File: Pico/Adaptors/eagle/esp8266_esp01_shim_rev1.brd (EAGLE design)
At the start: 17.1 x 10.7 mm, 4 parts, among them IC2 78L 3.3v

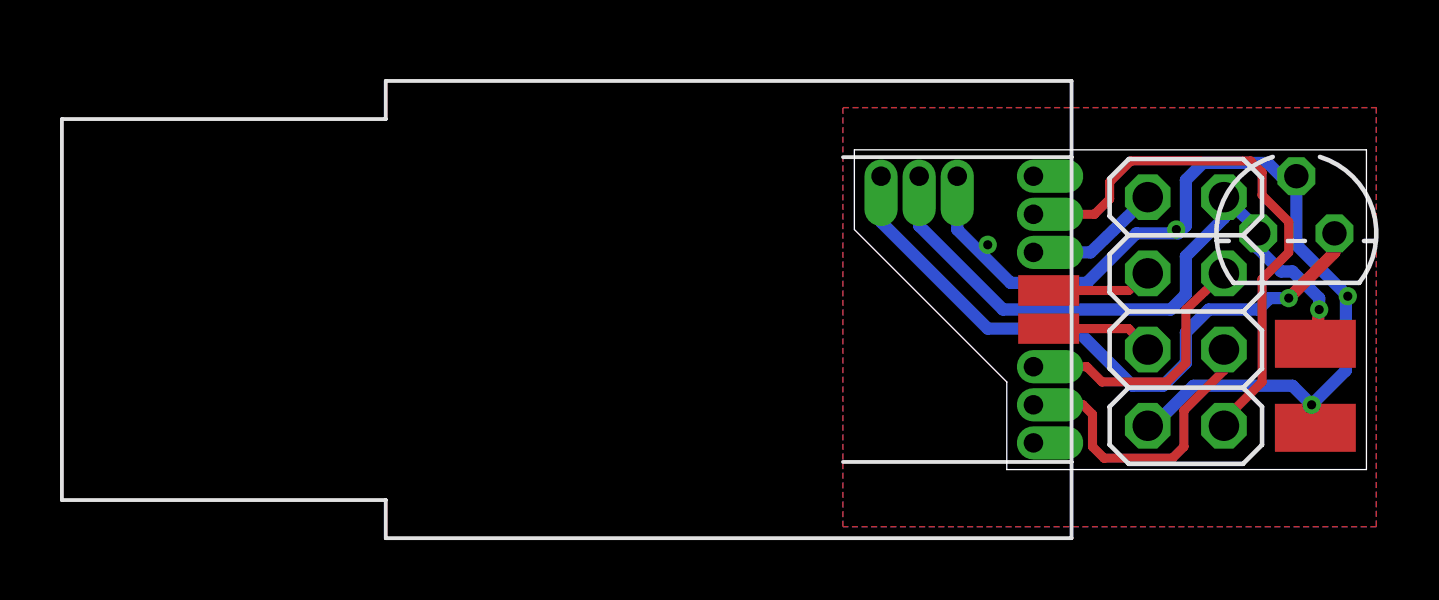
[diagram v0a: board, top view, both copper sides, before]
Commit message: tweak net classes
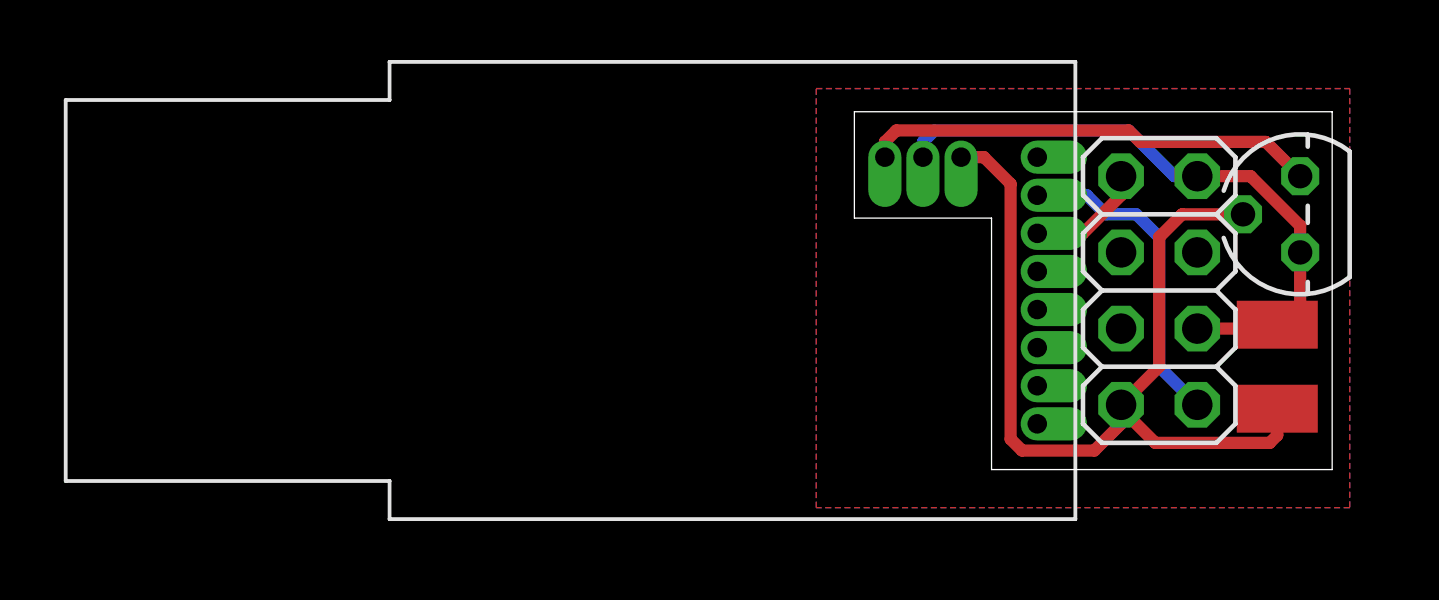
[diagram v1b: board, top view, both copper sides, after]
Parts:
- U$1: value ESPRUINO_PICO_0.05_SMALL -> ESPRUINO_PICO_0.05; device espruino_pico:ESPRUINO_PICO_0.05_SMALL -> espruino_pico:ESPRUINO_PICO_0.05
- moved C1 1.42 mm to (14.1, 3.43)
- moved U$1 1.31 mm to (-0.25, 5.97)
- moved ESP8266 1.13 mm to (10.2, 5.97)
- moved IC2 0.65 mm to (14.9, 8.51), turned to 90 degrees
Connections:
- removed net ESP_CH_PD: ESP8266.6, U$1.B9
- removed net ESP_GPIO0: ESP8266.3, U$1.A1
- removed net ESP_GPIO2: ESP8266.5, U$1.A0
- removed net ESP_RST: ESP8266.4, U$1.A10
- net VCC: now also ESP8266.6
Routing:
- net ESP_CH_PD: track 10.3 -> 0.00 mm
- net ESP_RST: track 9.08 -> 0.00 mm
- net ESP_TX: track 18.6 -> 10.8 mm
- net N$1: track 22.0 -> 15.1 mm, vias 1 -> 0
- net ESP_GPIO2: track 3.61 -> 0.00 mm
- net ESP_GPIO0: track 3.52 -> 0.00 mm
- net VCC: track 22.6 -> 21.0 mm, vias 1 -> 0
- net GND: track 32.4 -> 31.4 mm, vias 4 -> 0
- net ESP_RX: track 4.55 -> 3.96 mm
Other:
- board size 17.1 x 10.7 mm -> 15.9 x 11.9 mm
- board text removed: "3.3"
- board text removed: "47uF"
- board text removed: "GND"
- board text removed: "Vin"
